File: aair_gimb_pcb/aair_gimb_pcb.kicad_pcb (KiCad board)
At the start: 4 copper layers, 80.1 x 43 mm, 94 parts, among them J1 I2C, J2 UART, J3 USB_B_Mini, J5 SWD, J6 SPI1, Q1 sir182dp, Q2 sir182dp, Q3 sir182dp, Q4 sir182dp, Q5 sir182dp, Q6 sir182dp, U1 DRV8302, U2 STM32F405RGTx, U3 TC2117, U4 USBLC6-2SC6, X2 8MHz

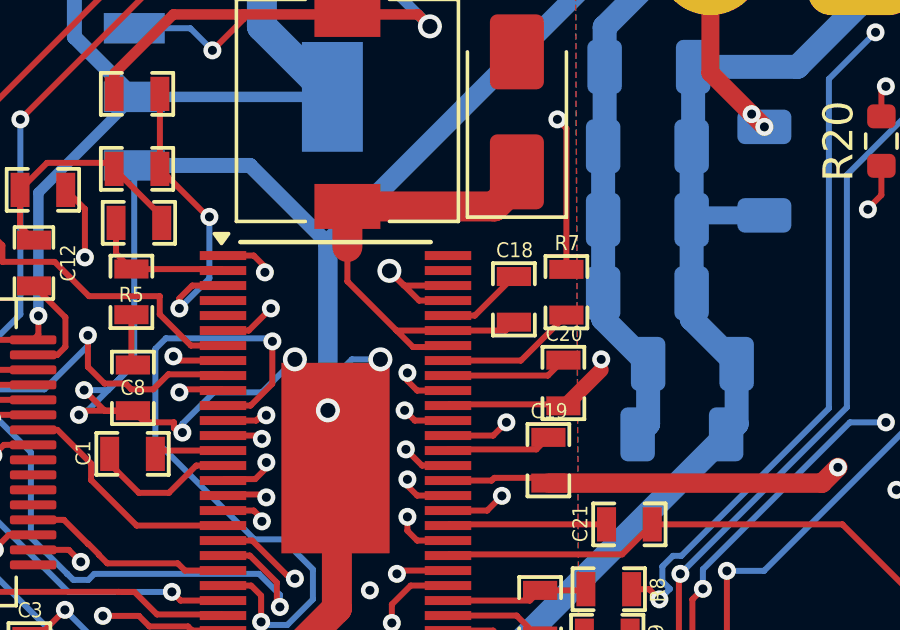
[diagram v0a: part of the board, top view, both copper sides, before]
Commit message: pcb, step
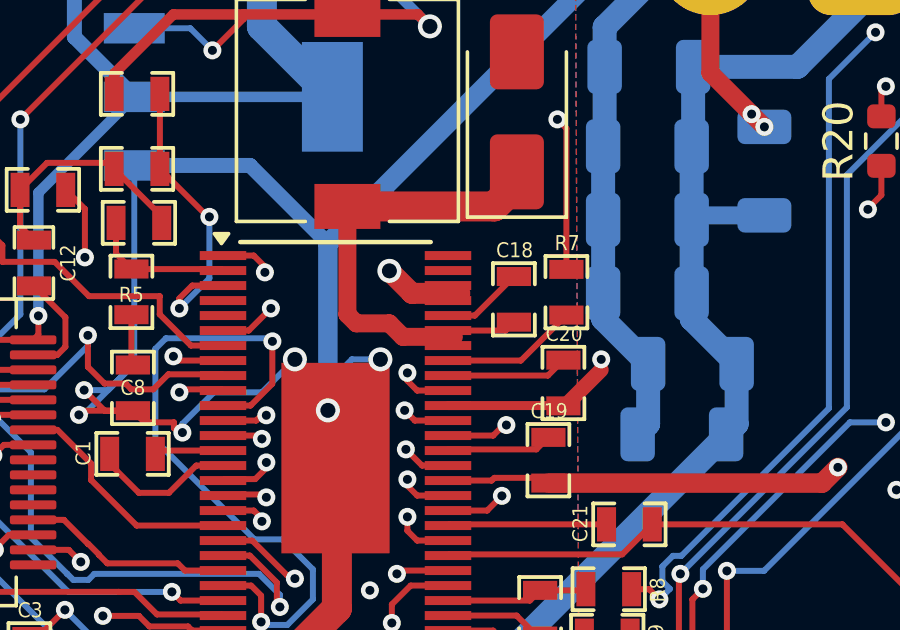
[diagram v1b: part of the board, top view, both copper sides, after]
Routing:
- net V_SUPPLY: track 83.3 -> 81.4 mm
- net Net-(D3-K): track 17.0 -> 16.1 mm
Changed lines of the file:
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@@
 			(outputformat 1)
 			(mirror no)
-			(drillshape 1)
+			(drillshape 0)
 			(scaleselection 1)
-			(outputdirectory "")
+			(outputdirectory "pcb/")
 		)
 	)
@@
 			)
 		)
+		(model "C:/Users/Gigabyte/Downloads/amass-xt30pw-m-_-pcb-solder-1.snapshot.2/Amass_XT30PW-M_pcb solder.stp"
+			(offset
+				(xyz -2.5 4 2.5)
+			)
+			(scale
+				(xyz 1 1 1)
+			)
+			(rotate
+				(xyz -0 -0 -180)
+			)
+		)
 	)
 	(footprint "CRF1:SMD-0603_r"
@@
 	)
 	(segment
-		(start 162.49 82.99)
-		(end 163.4534 82.99)
+		(start 163.4534 94.99)
+		(end 162.01 94.99)
 		(width 0.2)
 		(layer "F.Cu")
@@
 	)
 	(segment
-		(start 163.4534 94.99)
-		(end 162.01 94.99)
-		(width 0.2)
+		(start 161.5 82)
+		(end 162.25 82.75)
+		(width 0.7)
 		(layer "F.Cu")
 		(net 2)
@@
 	)
 	(segment
-		(start 161.5 82)
-		(end 162.49 82.99)
-		(width 0.2)
-		(layer "F.Cu")
-		(net 2)
-	)
-	(segment
 		(start 163.4534 94.99)
 		(end 163.4534 96.4534)
@@
 	)
 	(segment
-		(start 161.5 82)
-		(end 161.99 82.49)
-		(width 0.2)
+		(start 162.25 82.75)
+		(end 163.85 82.75)
+		(width 0.7)
 		(layer "F.Cu")
 		(net 2)
@@
 	)
 	(segment
-		(start 161.99 82.49)
-		(end 163.4534 82.49)
-		(width 0.2)
-		(layer "F.Cu")
-		(net 2)
-	)
-	(segment
 		(start 162.55 100.85)
 		(end 161.025 100.85)
@@
 	)
 	(segment
+		(start 160.1005 83.4505)
+		(end 160.4 83.75)
+		(width 0.6)
+		(layer "F.Cu")
+		(net 17)
+	)
+	(segment
 		(start 163.4534 84.49)
 		(end 163.4044 84.539)
@@
 	)
 	(segment
-		(start 165.372 83.99)
-		(end 163.4534 83.99)
-		(width 0.2)
+		(start 161.95 84.2)
+		(end 163.65 84.2)
+		(width 0.6)
 		(layer "F.Cu")
 		(net 17)
 	)
 	(segment
-		(start 160.1005 79.85278)
-		(end 160.1005 81.20597)
-		(width 1)
+		(start 161.5 83.75)
+		(end 161.95 84.2)
+		(width 0.6)
 		(layer "F.Cu")
 		(net 17)
 	)
 	(segment
-		(start 161.74 83.99)
-		(end 160.1005 82.3505)
+		(start 165.372 83.99)
+		(end 163.4534 83.99)
 		(width 0.2)
 		(layer "F.Cu")
@@
 	)
 	(segment
-		(start 163.4044 84.539)
-		(end 162.289 84.539)
-		(width 0.2)
-		(layer "F.Cu")
-		(net 17)
-	)
-	(segment
-		(start 160.1005 82.3505)
-		(end 160.1005 81.20597)
-		(width 0.2)
+		(start 160.1005 83.4505)
+		(end 160.1005 79.85278)
+		(width 0.6)
 		(layer "F.Cu")
 		(net 17)
 	)
 	(segment
-		(start 162.289 84.539)
-		(end 161.74 83.99)
-		(width 0.2)
+		(start 160.4 83.75)
+		(end 161.5 83.75)
+		(width 0.6)
 		(layer "F.Cu")
 		(net 17)
@@
 	)
 	(segment
-		(start 163.4534 83.99)
-		(end 161.74 83.99)
-		(width 0.2)
-		(layer "F.Cu")
-		(net 17)
-	)
-	(segment
 		(start 193.88 79.48)
 		(end 196.5 79.48)
@@
 	)
 	(segment
+		(start 167.29 86.49)
+		(end 167.3 86.5)
+		(width 0.2)
+		(layer "F.Cu")
+		(net 21)
+	)
+	(segment
 		(start 168.560659 84.95)
 		(end 168.56066 84.950001)
@@
 	)
 	(segment
+		(start 163.4534 86.49)
+		(end 167.29 86.49)
+		(width 0.3)
+		(layer "F.Cu")
+		(net 21)
+	)
+	(segment
 		(start 193.865 69.02)
 		(end 195.72 69.02)
@@
 	)
 	(segment
+		(start 163.4534 86.49)
+		(end 163.4944 86.449)
+		(width 0.2)
+		(layer "F.Cu")
+		(net 21)
+	)
+	(segment
 		(start 168.56066 85.30134)
 		(end 167.3 86.562)
@@
 	)
 	(segment
-		(start 163.4944 86.449)
-		(end 167.249 86.449)
-		(width 0.2)
-		(layer "F.Cu")
-		(net 21)
-	)
-	(segment
-		(start 167.249 86.449)
-		(end 167.3 86.5)
-		(width 0.2)
-		(layer "F.Cu")
-		(net 21)
-	)
-	(segment
-		(start 163.4534 86.49)
-		(end 163.4944 86.449)
-		(width 0.2)
-		(layer "F.Cu")
-		(net 21)
-	)
-	(segment
 		(start 190.45 75.6)
 		(end 190.45 74.315)
@@
 	)
 	(segment
+		(start 167.249 86.449)
+		(end 167.3 86.5)
+		(width 0.2)
+		(layer "F.Cu")
+		(net 21)
+	)
+	(segment
 		(start 195.72 69.02)
 		(end 197.635 70.935)
@@
 	)
 	(segment
-		(start 163.4534 87.49)
-		(end 164.96 87.49)
+		(start 169.574 92.612)
+		(end 170.162 92.612)
 		(width 0.2)
 		(layer "F.Cu")
@@
 	)
 	(segment
-		(start 169.574 92.612)
-		(end 170.162 92.612)
+		(start 165.2 87.25)
+		(end 164.96 87.49)
 		(width 0.2)
 		(layer "F.Cu")
@@
 	)
 	(segment
+		(start 164.96 87.49)
+		(end 163.4534 87.49)
+		(width 0.2)
+		(layer "F.Cu")
+		(net 67)
+	)
+	(segment
 		(start 177.9 75.99853)
 		(end 177.9 76.85)
@@
 	)
 	(segment
-		(start 164.96 87.49)
-		(end 165.4 87.05)
+		(start 165.29 87.25)
+		(end 165.2 87.25)
 		(width 0.2)
 		(layer "F.Cu")
@@
 	)
 	(segment
+		(start 165.4 87.14)
+		(end 165.29 87.25)
+		(width 0.2)
+		(layer "F.Cu")
+		(net 67)
+	)
+	(segment
 		(start 188.56 73.48)
 		(end 188.565 73.475)
@@
 	)
 	(via
-		(at 165.4 87.05)
+		(at 165.4 87.14)
 		(size 0.6)
 		(drill 0.3)
@@
 	)
 	(segment
-		(start 187.15 76.3)
-		(end 187.15 73.48)
+		(start 184.9 78.55)
+		(end 187.15 76.3)
 		(width 0.5)
 		(layer "In2.Cu")
@@
 	)
 	(segment
-		(start 165.4 87.05)
-		(end 173.9 78.55)
+		(start 165.4 87.14)
+		(end 165.4 87.05)
 		(width 0.5)
 		(layer "In2.Cu")
@@
 	)
 	(segment
-		(start 184.9 78.55)
-		(end 187.15 76.3)
+		(start 187.15 76.3)
+		(end 187.15 73.48)
 		(width 0.5)
 		(layer "In2.Cu")
@@
 		(layer "In2.Cu")
 		(net 67)
+	)
+	(segment
+		(start 165.4 87.05)
+		(end 173.9 78.55)
+		(width 0.5)
+		(layer "In2.Cu")
+		(net 67)
